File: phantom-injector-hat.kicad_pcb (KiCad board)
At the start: 2 copper layers, 65 x 44.8 mm, 42 parts, among them J1 Conn_02x20_Odd_Even, J2 Conn_02x03_Top_Bottom, J3 Conn_01x03, J4 Conn_01x03, SW1 SW_SPST, U1 LT8362EMSE-PBF

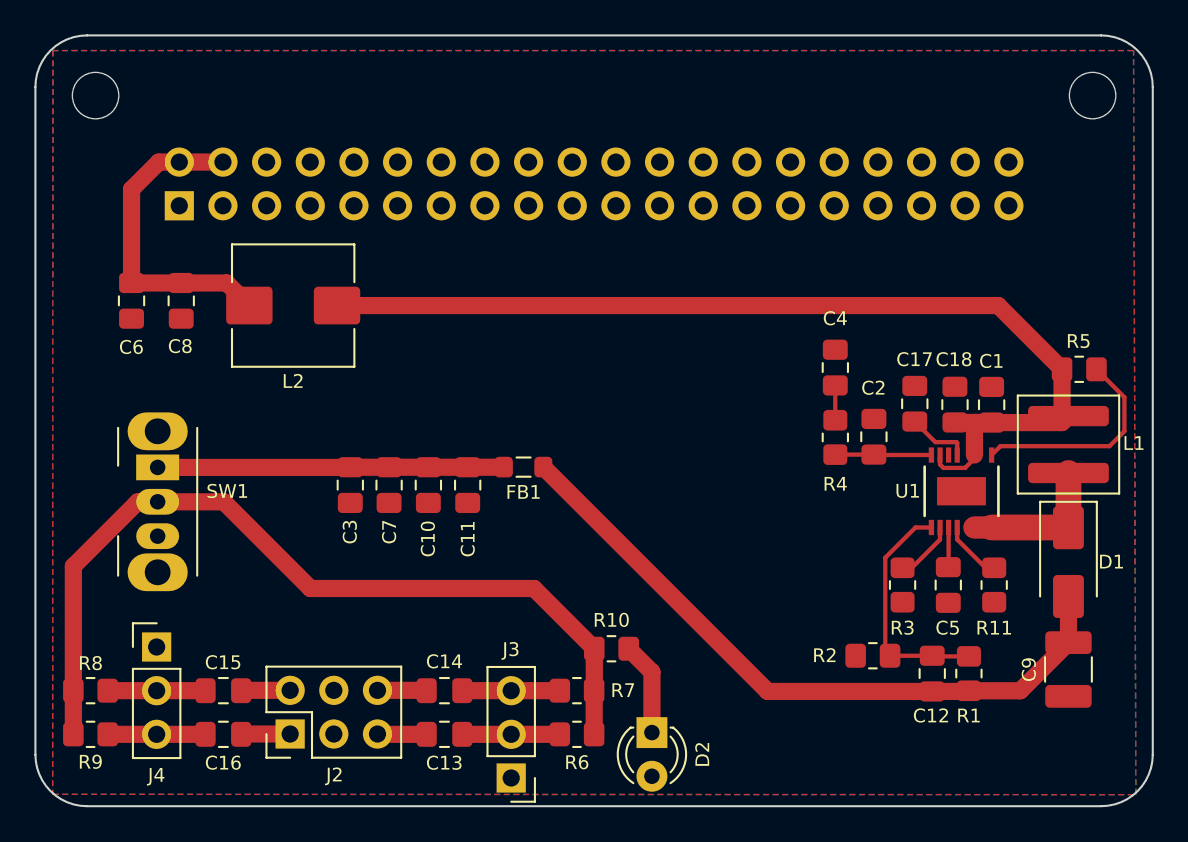
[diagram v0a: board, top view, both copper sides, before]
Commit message: WIP
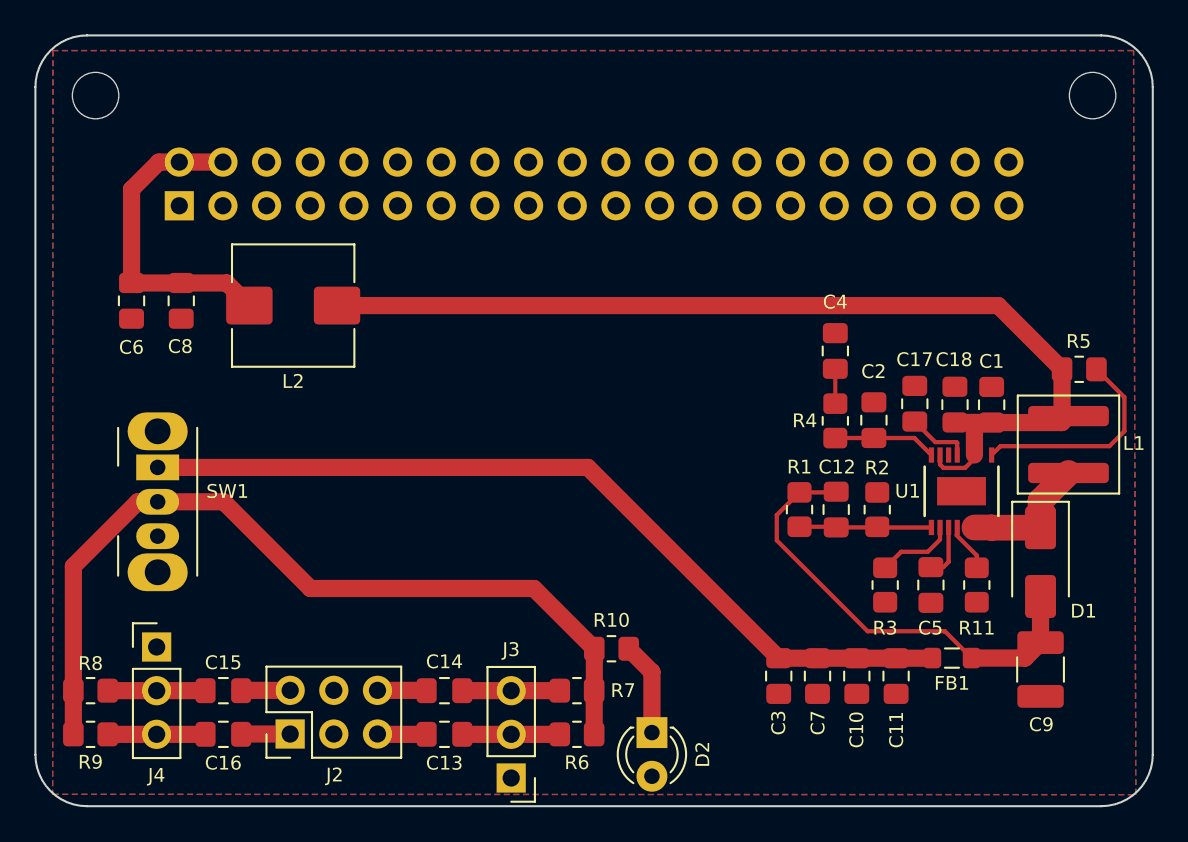
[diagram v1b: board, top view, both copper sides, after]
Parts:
- moved C10 27.3 mm to (147.8, 81.3)
- moved C11 27.3 mm to (150.1, 81.3)
- moved C7 27.3 mm to (145.5, 81.3)
- moved C3 27.3 mm to (143.2, 81.3)
- moved FB1 27.3 mm to (153.3, 80.2)
- moved R1 13.7 mm to (144.4, 71.6), turned to -90 degrees
- moved C12 11.1 mm to (146.6, 71.6), turned to -90 degrees
- moved R2 8.50 mm to (149.0, 71.6), turned to 90 degrees
- moved C9 1.63 mm to (158.5, 80.9)
- moved D1 1.63 mm to (158.5, 74.6)
- moved C5 1.01 mm to (152.1, 76.0)
- moved R11 1.01 mm to (154.8, 76.0)
- moved R3 1.01 mm to (149.4, 76.0)
- moved C4 0.97 mm to (146.5, 62.4)
- moved C2 0.97 mm to (148.8, 66.4)
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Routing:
- net /+48V: track 20.1 -> 49.7 mm
- net /+48V_RAW: track 39.8 -> 26.7 mm
- net /FBX: track 13.8 -> 7.72 mm
- net /SYNC_MODE: track 3.53 -> 2.39 mm
- net /RT: track 3.56 -> 4.58 mm
- net /SW_NODE: track 8.66 -> 7.71 mm
- net /SS: track 2.32 -> 3.16 mm

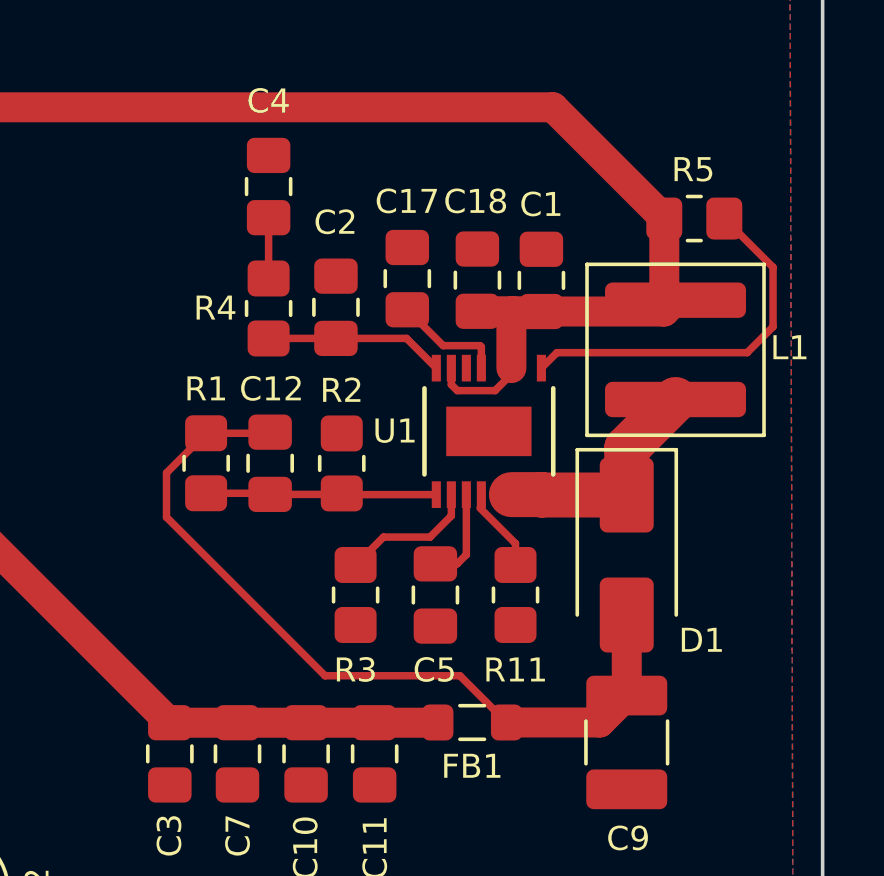
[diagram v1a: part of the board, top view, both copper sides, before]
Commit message: Chkpt
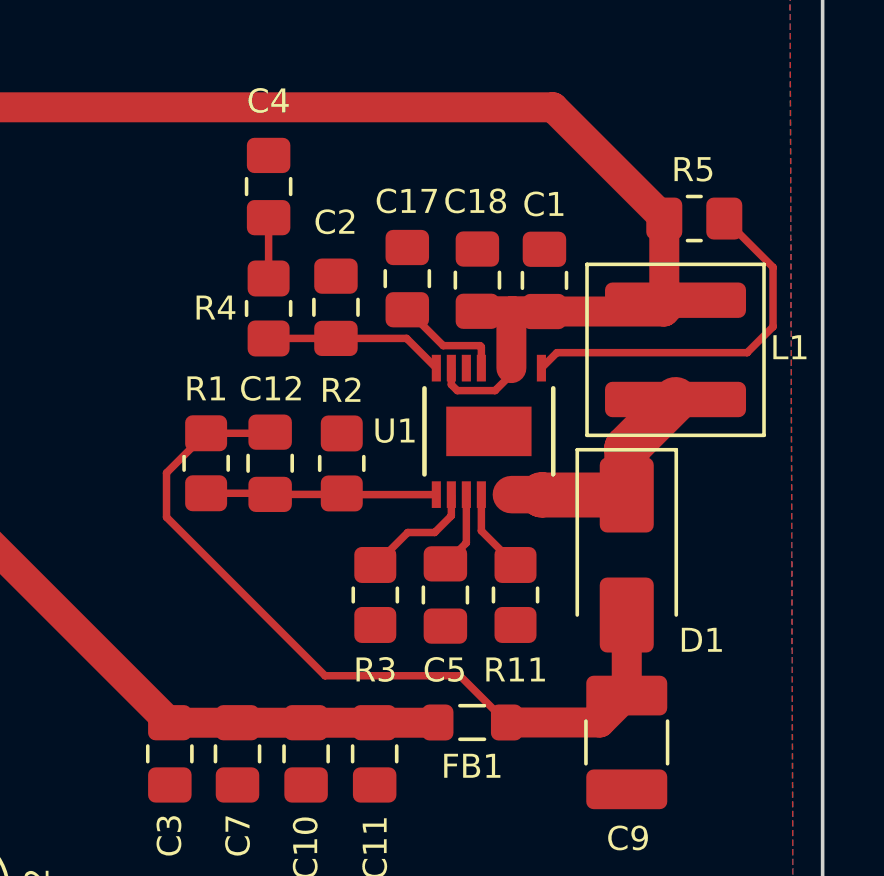
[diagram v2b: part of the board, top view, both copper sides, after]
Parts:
- moved R3 0.66 mm to (150.1, 76.0)
- moved C5 0.33 mm to (152.4, 76.0)
- moved C1 0.10 mm to (155.7, 65.5)
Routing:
- net /RT: track 4.58 -> 3.92 mm
- net /SS: track 3.16 -> 2.60 mm
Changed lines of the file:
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@@
 	(footprint "Capacitor_SMD:C_0805_2012Metric_Pad1.18x1.45mm_HandSolder"
 		(layer "F.Cu")
-		(at 152.0924 75.9716 -90)
+		(at 152.4256 75.9716 -90)
 		(descr "Capacitor SMD 0805 (2012 Metric), square (rectangular) end terminal, IPC-7351 nominal with elongated pad for handsoldering. (Body size source: IPC-SM-782 page 76, https://www.pcb-3d.com/wordpress/wp-content/uploads/ipc-sm-782a_amendment_1_and_2.pdf, https://docs.google.com/spreadsheets/d/1BsfQQcO9C6DZCsRaXUlFlo91Tg2WpOkGARC1WS5S8t0/edit?usp=sharing)")
 		(tags "capacitor handsolder")
@@
 	(footprint "Resistor_SMD:R_0805_2012Metric_Pad1.20x1.40mm_HandSolder"
 		(layer "F.Cu")
-		(at 149.4324 75.9716 -90)
+		(at 150.0888 75.9716 -90)
 		(descr "Resistor SMD 0805 (2012 Metric), square (rectangular) end terminal, IPC-7351 nominal with elongated pad for handsoldering. (Body size source: IPC-SM-782 page 72, https://www.pcb-3d.com/wordpress/wp-content/uploads/ipc-sm-782a_amendment_1_and_2.pdf)")
 		(tags "resistor handsolder")
@@
 	(footprint "Capacitor_SMD:C_0805_2012Metric_Pad1.18x1.45mm_HandSolder"
 		(layer "F.Cu")
-		(at 155.626 65.4853 90)
+		(at 155.7276 65.4853 90)
 		(descr "Capacitor SMD 0805 (2012 Metric), square (rectangular) end terminal, IPC-7351 nominal with elongated pad for handsoldering. (Body size source: IPC-SM-782 page 76, https://www.pcb-3d.com/wordpress/wp-content/uploads/ipc-sm-782a_amendment_1_and_2.pdf, https://docs.google.com/spreadsheets/d/1BsfQQcO9C6DZCsRaXUlFlo91Tg2WpOkGARC1WS5S8t0/edit?usp=sharing)")
 		(tags "capacitor handsolder")
@@
 	)
 	(segment
-		(start 153.12413 74.62737)
-		(end 153.12413 72.6264)
+		(start 153.12413 72.6264)
+		(end 153.12413 74.23557)
 		(width 0.25)
 		(layer "F.Cu")
@@
 	)
 	(segment
-		(start 152.0924 74.9341)
-		(end 152.8174 74.9341)
-		(width 0.25)
-		(layer "F.Cu")
-		(net "/SS")
-	)
-	(segment
-		(start 152.8174 74.9341)
-		(end 153.12413 74.62737)
+		(start 153.12413 74.23557)
+		(end 152.4256 74.9341)
 		(width 0.25)
 		(layer "F.Cu")
@@
 	)
 	(segment
-		(start 154.7624 74.9716)
-		(end 154.7624 74.255555)
+		(start 153.62451 73.83371)
+		(end 154.7624 74.9716)
 		(width 0.25)
 		(layer "F.Cu")
@@
 	)
 	(segment
-		(start 154.7624 74.255555)
-		(end 153.58153 73.074685)
+		(start 153.62451 72.6264)
+		(end 153.62451 73.83371)
 		(width 0.25)
 		(layer "F.Cu")
@@
 	)
 	(segment
-		(start 152.62375 72.6264)
+		(start 152.06787 73.8888)
 		(end 152.62375 73.33292)
 		(width 0.25)
@@
 	)
 	(segment
-		(start 151.91507 74.0416)
-		(end 150.3624 74.0416)
+		(start 152.62375 73.33292)
+		(end 152.62375 72.6264)
 		(width 0.25)
 		(layer "F.Cu")
@@
 	)
 	(segment
-		(start 152.62375 73.33292)
-		(end 151.91507 74.0416)
+		(start 151.1716 73.8888)
+		(end 152.06787 73.8888)
 		(width 0.25)
 		(layer "F.Cu")
@@
 	)
 	(segment
-		(start 150.3624 74.0416)
-		(end 149.4324 74.9716)
+		(start 150.0888 74.9716)
+		(end 151.1716 73.8888)
 		(width 0.25)
 		(layer "F.Cu")
@@
 	)
 	(segment
-		(start 155.626 72.6264)
-		(end 154.62524 72.6264)
-		(width 1.5)
+		(start 154.62527 72.6264)
+		(end 155.626 72.6264)
+		(width 1.25)
 		(layer "F.Cu")
 		(net "/SW_NODE")
